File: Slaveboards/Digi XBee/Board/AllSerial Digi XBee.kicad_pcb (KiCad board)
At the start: 2 copper layers, 67.4 x 44.8 mm, 2 parts, among them X1 AllSerial Slaveboard

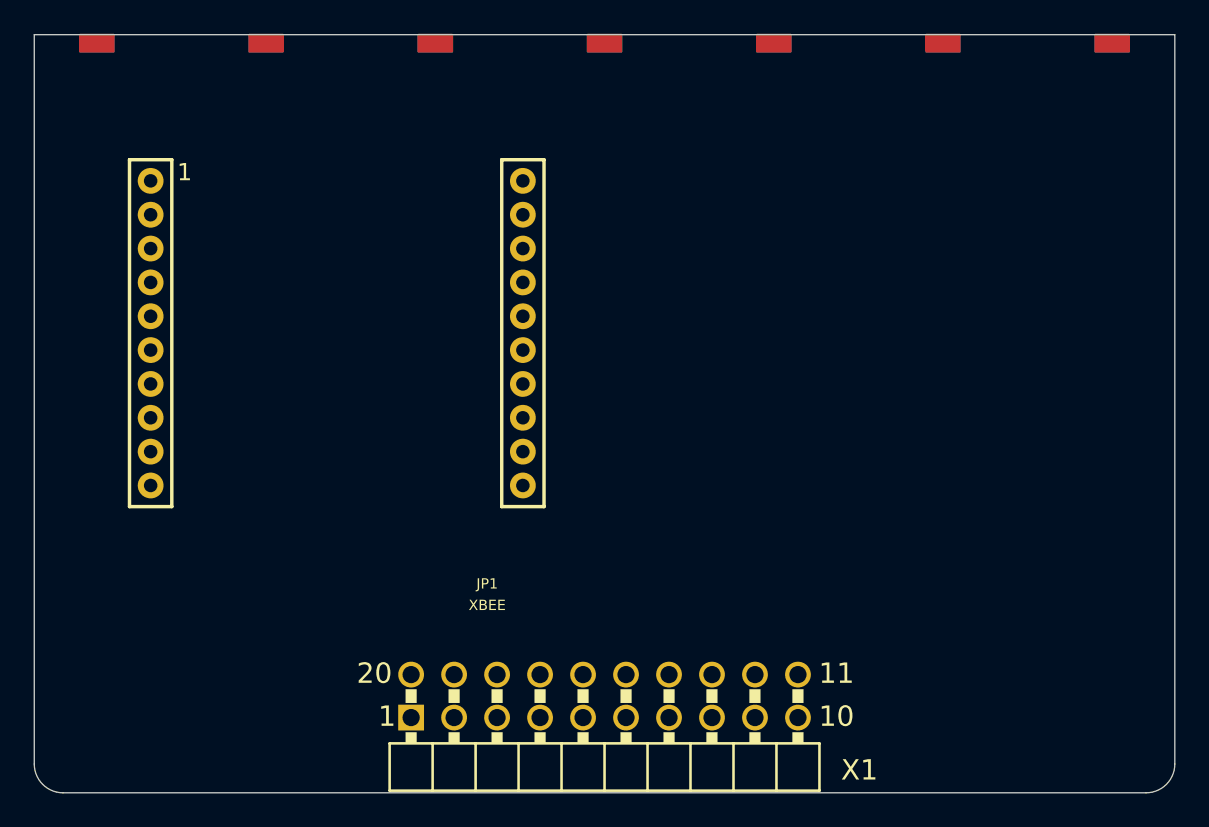
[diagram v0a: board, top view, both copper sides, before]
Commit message: Added new boards
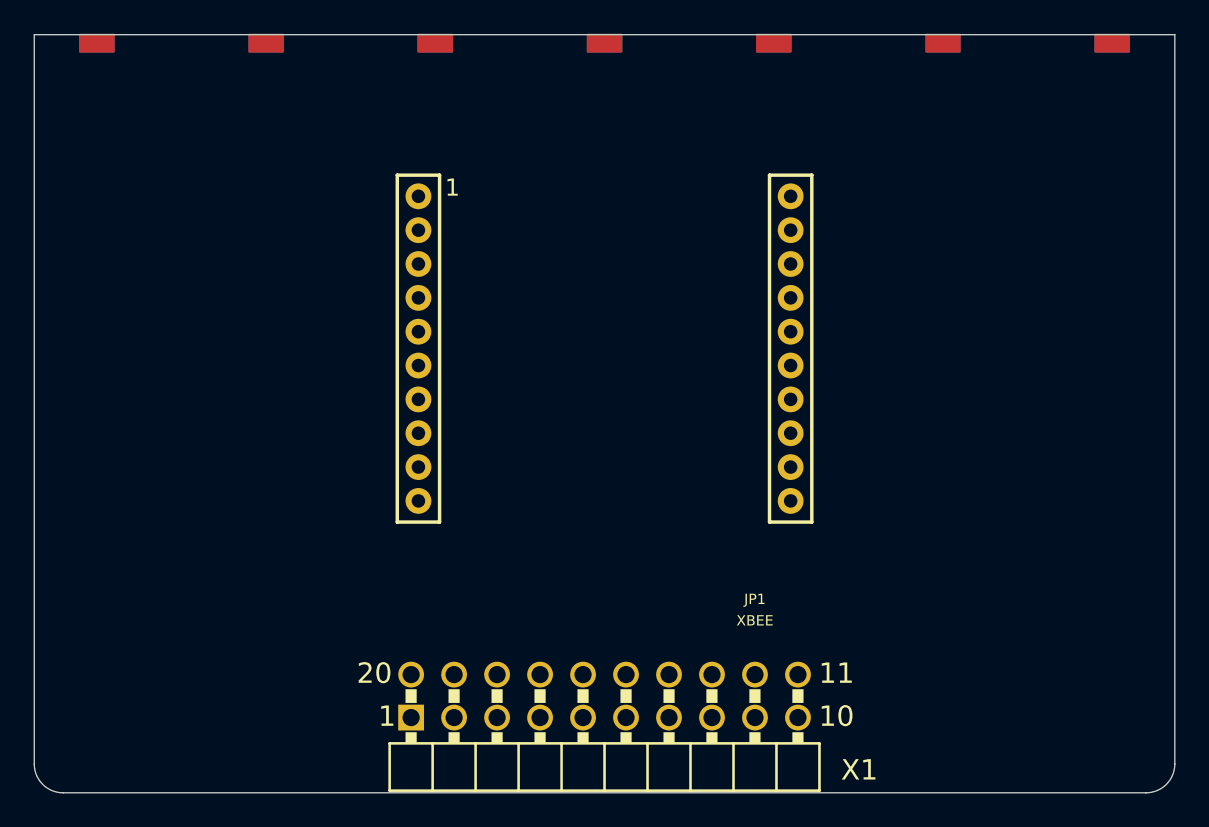
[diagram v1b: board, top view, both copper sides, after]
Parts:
- moved JP1 15.9 mm to (173.0, 111.6)
